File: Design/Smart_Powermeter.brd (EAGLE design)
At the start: 92 x 87 mm, 37 parts, among them J1 AUDIO_JACK_TRRSSMD_RA, J2 AUDIO_JACK_TRRSSMD_RA, J3 AUDIO_JACK_TRRSSMD_RA, J4 AUDIO_JACK_TRRSSMD_RA, J5 AUDIO_JACK_TRRSSMD_RA, J6 AUDIO_JACK_TRRSSMD_RA, J7 AUDIO_JACK_TRRSSMD_RA

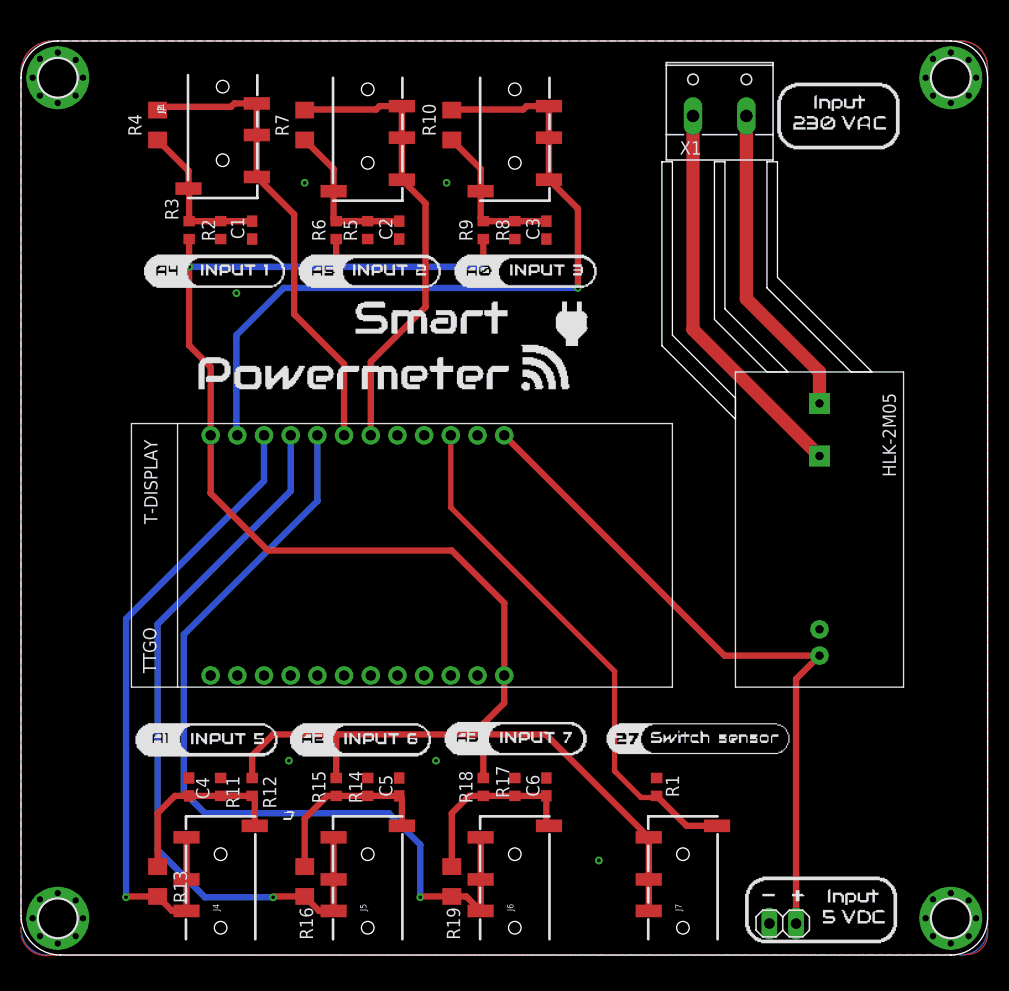
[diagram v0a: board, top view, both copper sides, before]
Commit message: Added design files of V2
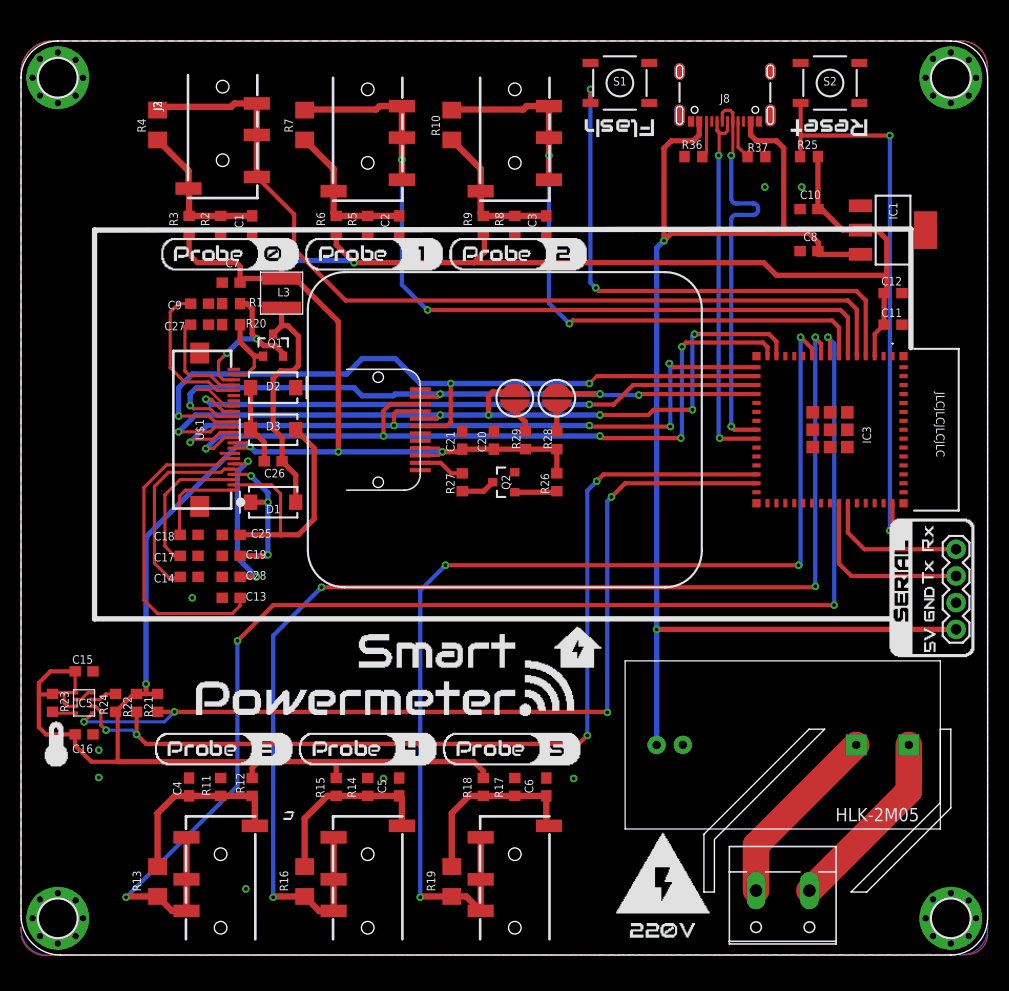
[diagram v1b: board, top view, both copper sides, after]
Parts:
- removed JP1: (no value), pinhead:1X02
- added C10, C12, C16, C20, C8: 10uF, rcl:C0603
- added C11, C15, C21: 0.1uF, rcl:C0603
- added C13, C14, C17, C18, C19, C25, C27, C28, C9: 1uF, rcl:C0603
- added C26, C7: 4.7uF, rcl:C0603
- added D1, D2, D3: SS14, SpaceDIY_semiconductors:SMA-DIODE
- added DISP1: DISP_LCD_GENERIC_SPI_1.69_WRAPUNDER, adafruit_display:TFT_1.69IN_240X280_12P
- added IC1: AMS1117-3.3, SparkFun-IC-Power:SOT223
- added IC3: ESP32-S2-MINI-1-N4R2, SpaceDIY_modules:ESP32S2MINI1N4R2
- added IC5: BMP280, SamacSys_Parts:8-PIN-METAL-LID-LGA
- added J8: USB-C, SparkFun-Connectors:USB-C-16P-4LAYER-ISOLATED
- added L3: 10uH, microbuilder:INDUCTOR_4X4MM_NR401
- added Q1: IRLML0100, Parts:SOT23-3
- added Q2: 2N7002, SparkFun-DiscreteSemi:SOT23-3
- added R20, R21, R22, R26, R28, R29: 10k, rcl:R0603
- added R23, R24: 4.7k, rcl:R0603
- added R25: 10K, rcl:R0603
- added R27: 10, rcl:R0603
- added R36, R37: 5.1k, rcl:R0603
- added S1: Flash, SpaceDIY_electromechanical:TACTILE_SWITCH_SMD_5.2MM
- added S2: Reset, SpaceDIY_electromechanical:TACTILE_SWITCH_SMD_5.2MM
- added SJ1, SJ2: SOLDERJUMPERROUND, SparkFun-Retired:SJ_ROUND
- H1: value (none) -> 92X84
- J7: value AUDIO_JACK_TRRSSMD_RA -> (none); device SparkFun-Connectors:AUDIO_JACK_3.5MM_TRRS_SMD_RA -> SparkFun-Connectors:1X04
- R1: value 10k -> 0.47
- U$1: value TTGO-T-DISPLAYFRAME -> E-PAPER-FPC_2; device TTGO-TDisplay:TTGO-T-DISPLAY-OL -> SpaceDIY_connectors:FPC-05FB-24PH20
- moved X1 75.2 mm to (72.5, 5.50), turned to 180 degrees
- moved R1 61.3 mm to (20.0, 62.0), turned to 180 degrees
- moved U$1 51.2 mm to (17.0, 50.0), turned to 270 degrees
- moved J7 39.7 mm to (89.0, 31.0)
- moved U$2 33.7 mm to (87.5, 28.0), turned to 180 degrees
- moved C1 0.50 mm to (22.0, 69.5)
- moved C2 0.50 mm to (36.0, 69.5)
- moved C3 0.50 mm to (50.0, 69.5)
- moved R2 0.50 mm to (19.0, 69.5)
- moved R3 0.50 mm to (16.0, 69.5)
- moved R5 0.50 mm to (33.0, 69.5)
- moved R6 0.50 mm to (30.0, 69.5)
- moved R8 0.50 mm to (47.0, 69.5)
- moved R9 0.50 mm to (44.0, 69.5)
- renumbered FRAME1 to H1
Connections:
- removed net M6: J6.RING1, J6.RING2, J6.TIP, R19.2, U$1.SVN-G39-A3
- removed net PB: J7.EARTH, R1.2, U$1.27-G27-A17
- removed net VG6: C6.1, J6.EARTH, R17.2, R18.1, R19.1
- new net BK_LIGHT: Q2.1, R26.1
- new net CC3: J8.B5, R36.2
- new net CC4: J8.A5, R37.2
- new net D+: IC3.24, J8.A6, J8.B6
- new net D-: IC3.23, J8.A7, J8.B7
- new net GDR: Q1.1, R20.1, U$1.23
- new net IO0: IC3.4, S1.3
- new net LEDK: DISP1.2, R27.2
- new net M0: IC3.5, J1.RING1, J1.RING2, J1.TIP, R4.2
- new net N$10: IC5.5, R23.2
- new net N$11: C9.2, U$1.20
- new net N$12: C13.2, U$1.7
- new net N$13: C14.2, U$1.5
- new net N$14: C17.2, U$1.3
- new net N$15: C18.2, U$1.1
- new net N$16: C26.2, D2.A, D3.C
- new net N$17: C26.1, D1.A, L3.P$1, Q1.3
- new net N$3: IC5.2, R24.2
- new net N$31: C27.2, U$1.21
- new net N$32: C28.2, U$1.6
- new net N$4: Q2.3, R27.1
- new net N$5: R28.1, SJ1.2
- new net N$6: R29.1, SJ2.2
- new net RESE: Q1.2, R1.1, U$1.22
- new net RST: IC3.45, R25.1, S2.3
- new net RX: IC3.40, J7.4
- new net SCL: IC3.29, IC5.4, R21.2
- new net SDA: IC3.28, IC5.3, R22.2
- new net SPI_BUSY: IC3.18, U$1.16
- new net SPI_CLK: DISP1.9, IC3.16, U$1.12
- new net SPI_CS: DISP1.8, IC3.14, SJ2.1, U$1.13
- new net SPI_MISO: DISP1.7, IC3.17, U$1.14
- new net SPI_MOSI: DISP1.10, IC3.15, U$1.11
- new net SPI_RST: DISP1.11, IC3.19, SJ1.1, U$1.15
- new net TX: IC3.39, J7.3
- new net VG0: C1.1, J1.EARTH, R2.2, R3.1, R4.1
- new net VGH: C19.1, D1.C, U$1.4
- new net VGL: C25.1, D3.A, U$1.2
- net 3.3V: now also C10.1, C11.1, C12.1, C15.1, C16.1, C20.1, C21.1, C7.1, DISP1.3, DISP1.4, IC1.2, IC3.3, IC5.6, IC5.8, L3.P$2, R21.1, R22.1, R23.1, R24.1, R25.2, R26.2, R28.2, R29.2, U$1.10, U$1.9; no longer J7.RING1, J7.RING2, J7.TIP, U$1.3V3_0, U$1.3V3_1
- net 5V: now also C8.1, IC1.3, J7.1, J8.VBUS1, J8.VBUS2; no longer JP1.2, U$1.5V
- net GND: now also C10.2, C11.2, C12.2, C13.1, C14.1, C15.2, C16.2, C17.1, C18.1, C19.2, C20.2, C21.2, C25.2, C27.1, C28.1, C7.2, C8.2, C9.1, D2.C, DISP1.1, DISP1.12, DISP1.5, DISP1.6, H1.B3,1, H1.B3,2, H1.B3,3, H1.B3,6, H1.P$1, H1.P$10, H1.P$11, H1.P$12, H1.P$13, H1.P$14, H1.P$15, H1.P$16, H1.P$17, H1.P$18, H1.P$19, H1.P$2, H1.P$20, H1.P$21, H1.P$22, H1.P$23, H1.P$24, H1.P$25, H1.P$26, H1.P$27, H1.P$28, H1.P$29, H1.P$3, H1.P$30, H1.P$31, H1.P$32, H1.P$4, H1.P$5, H1.P$6, H1.P$7, H1.P$8, H1.P$9, IC1.1, IC3.1, IC3.2, IC3.30, IC3.42, IC3.43, IC3.46, IC3.47, IC3.48, IC3.49, IC3.50, IC3.51, IC3.52, IC3.53, IC3.54, IC3.55, IC3.56, IC3.57, IC3.58, IC3.59, IC3.60, IC3.61, IC3.62, IC3.63, IC3.64, IC3.65, IC3.66, IC3.67, IC3.68, IC3.69, IC3.70, IC3.71, IC3.72, IC3.73, IC5.1, IC5.7, J7.2, J8.GND, J8.GND2, Q2.2, R1.2, R20.2, R36.1, R37.1, S1.1, S2.1, U$1.17, U$1.8; no longer JP1.1, R1.1, U$1.GND_0, U$1.GND_1, U$1.GND_2, U$1.GND_3, U$1.GND_4
- net M1: now also IC3.6, J2.RING1, J2.RING2, J2.TIP, R7.2; no longer J1.RING1, J1.RING2, J1.TIP, R4.2, U$1.32-G32-A4
- net M2: now also IC3.7, J3.RING1, J3.RING2, J3.TIP, R10.2; no longer J2.RING1, J2.RING2, J2.TIP, R7.2, U$1.33-G33-A5
- net M3: now also IC3.8, J4.RING1, J4.RING2, J4.TIP, R13.2; no longer J3.RING1, J3.RING2, J3.TIP, R10.2, U$1.SVP-G36-A0
- net M4: now also IC3.9, J5.RING1, J5.RING2, J5.TIP, R16.2; no longer J4.RING1, J4.RING2, J4.TIP, R13.2, U$1.37-G37
- net M5: now also IC3.10, J6.RING1, J6.RING2, J6.TIP, R19.2; no longer J5.RING1, J5.RING2, J5.TIP, R16.2, U$1.38-G38
- net N$1: now also U$2.AC2; no longer U$2.AC1
- net N$2: now also U$2.AC1; no longer U$2.AC2
- net VG1: now also C2.1, J2.EARTH, R5.2, R6.1, R7.1; no longer C1.1, J1.EARTH, R2.2, R3.1, R4.1
- net VG2: now also C3.1, J3.EARTH, R10.1, R8.2, R9.1; no longer C2.1, J2.EARTH, R5.2, R6.1, R7.1
- net VG3: now also C4.1, J4.EARTH, R11.2, R12.1, R13.1; no longer C3.1, J3.EARTH, R10.1, R8.2, R9.1
- net VG4: now also C5.1, J5.EARTH, R14.2, R15.1, R16.1; no longer C4.1, J4.EARTH, R11.2, R12.1, R13.1
- net VG5: now also C6.1, J6.EARTH, R17.2, R18.1, R19.1; no longer C5.1, J5.EARTH, R14.2, R15.1, R16.1
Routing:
- net 3.3V: track 164.0 -> 265.6 mm, vias 3 -> 6
- net SDA: track 0.00 -> 91.8 mm, vias 0 -> 4
- net SCL: track 0.00 -> 88.0 mm, vias 0 -> 4
- net M0: track 0.00 -> 85.4 mm
- net M6: track 82.2 -> 0.00 mm, vias 1 -> 0
- net SPI_CS: track 0.00 -> 78.7 mm, vias 0 -> 6
- net SPI_MOSI: track 0.00 -> 73.1 mm, vias 0 -> 5
- net SPI_MISO: track 0.00 -> 72.3 mm, vias 0 -> 3
- net SPI_CLK: track 0.00 -> 69.1 mm, vias 0 -> 5
- net SPI_RST: track 0.00 -> 66.5 mm, vias 0 -> 4
- net 5V: track 65.1 -> 124.5 mm, vias 0 -> 2
- net SPI_BUSY: track 0.00 -> 56.5 mm, vias 0 -> 2
- net M3: track 71.8 -> 128.0 mm, vias 1 -> 4
- net M4: track 62.8 -> 117.5 mm, vias 1 -> 4
- net RST: track 0.00 -> 53.9 mm, vias 0 -> 2
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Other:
- board text added: "JLCJLCJLCJLC"

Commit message: Updated design files
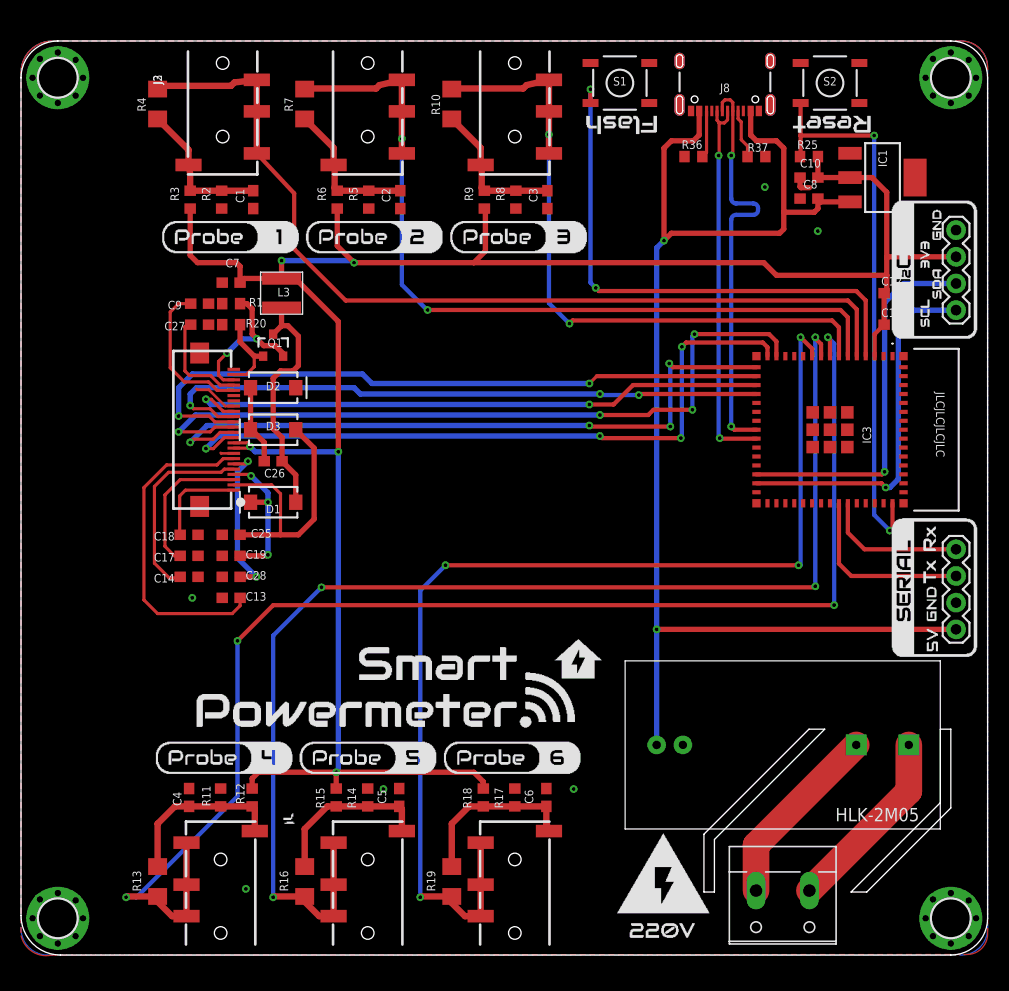
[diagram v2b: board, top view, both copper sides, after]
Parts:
- removed C15, C21: 0.1uF, rcl:C0603
- removed C16, C20: 10uF, rcl:C0603
- removed DISP1: DISP_LCD_GENERIC_SPI_1.69_WRAPUNDER, adafruit_display:TFT_1.69IN_240X280_12P
- removed IC5: BMP280, SamacSys_Parts:8-PIN-METAL-LID-LGA
- removed Q2: 2N7002, SparkFun-DiscreteSemi:SOT23-3
- removed R21, R22, R26, R28, R29: 10k, rcl:R0603
- removed R23, R24: 4.7k, rcl:R0603
- removed R27: 10, rcl:R0603
- removed SJ1, SJ2: SOLDERJUMPERROUND, SparkFun-Retired:SJ_ROUND
- added J9: (no value), SparkFun-Connectors:1X04
- moved IC1 5.10 mm to (82.0, 74.0)
- moved C8 5.00 mm to (75.0, 72.0)
- moved C10 3.00 mm to (75.0, 74.0)
- moved J2 2.50 mm to (33.0, 86.5)
- moved J3 2.50 mm to (47.0, 86.5)
- moved C1 2.40 mm to (22.1, 71.9)
- moved C2 2.40 mm to (36.1, 71.9)
- moved C3 2.40 mm to (50.1, 71.9)
- moved R2 2.40 mm to (19.1, 71.9)
- moved R3 2.40 mm to (16.1, 71.9)
- moved R5 2.40 mm to (33.1, 71.9)
- moved R6 2.40 mm to (30.1, 71.9)
- moved R8 2.40 mm to (47.1, 71.9)
- moved R9 2.40 mm to (44.1, 71.9)
- moved J1 2.25 mm to (19.2, 86.5)
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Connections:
- removed net BK_LIGHT: Q2.1, R26.1
- removed net LEDK: DISP1.2, R27.2
- removed net M0: IC3.5, J1.RING1, J1.RING2, J1.TIP, R4.2
- removed net N$10: IC5.5, R23.2
- removed net N$3: IC5.2, R24.2
- removed net N$4: Q2.3, R27.1
- removed net N$5: R28.1, SJ1.2
- removed net N$6: R29.1, SJ2.2
- new net M6: IC3.10, J6.RING1, J6.RING2, J6.TIP, R19.2
- net 3.3V: now also J9.2; no longer C15.1, C16.1, C20.1, C21.1, DISP1.3, DISP1.4, IC5.6, IC5.8, R21.1, R22.1, R23.1, R24.1, R26.2, R28.2, R29.2
- net GND: now also J9.1; no longer C15.2, C16.2, C20.2, C21.2, DISP1.1, DISP1.12, DISP1.5, DISP1.6, IC5.1, IC5.7, Q2.2
- net M1: now also IC3.5, J1.RING1, J1.RING2, J1.TIP, R4.2; no longer IC3.6, J2.RING1, J2.RING2, J2.TIP, R7.2
- net M2: now also IC3.6, J2.RING1, J2.RING2, J2.TIP, R7.2; no longer IC3.7, J3.RING1, J3.RING2, J3.TIP, R10.2
- net M3: now also IC3.7, J3.RING1, J3.RING2, J3.TIP, R10.2; no longer IC3.8, J4.RING1, J4.RING2, J4.TIP, R13.2
- net M4: now also IC3.8, J4.RING1, J4.RING2, J4.TIP, R13.2; no longer IC3.9, J5.RING1, J5.RING2, J5.TIP, R16.2
- net M5: now also IC3.9, J5.RING1, J5.RING2, J5.TIP, R16.2; no longer IC3.10, J6.RING1, J6.RING2, J6.TIP, R19.2
- net SCL: now also J9.4; no longer IC5.4, R21.2
- net SDA: now also J9.3; no longer IC5.3, R22.2
- net SPI_CLK: no longer DISP1.9
- net SPI_CS: no longer DISP1.8, SJ2.1
- net SPI_MISO: no longer DISP1.7
- net SPI_MOSI: no longer DISP1.10
- net SPI_RST: no longer DISP1.11, SJ1.1
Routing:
- net M6: track 0.00 -> 104.3 mm, vias 0 -> 4
- net M0: track 85.4 -> 0.00 mm
- net M3: track 128.0 -> 64.1 mm, vias 4 -> 2
- net 3.3V: track 265.6 -> 206.4 mm, vias 6 -> 5
- net SDA: track 91.8 -> 36.0 mm, vias 4 -> 1
- net SCL: track 88.0 -> 34.7 mm, vias 4 -> 1
- net M2: track 62.0 -> 77.8 mm
- net M5: track 103.7 -> 118.0 mm
- net M1: track 75.7 -> 87.6 mm, vias 2 -> 0
- net M4: track 117.5 -> 129.1 mm
- net SPI_MISO: track 72.3 -> 64.4 mm, vias 3 -> 2
- net SPI_CS: track 78.7 -> 72.0 mm, vias 6 -> 4
- net SPI_RST: track 66.5 -> 60.2 mm, vias 4 -> 3
- net SPI_MOSI: track 73.1 -> 67.0 mm, vias 5 -> 4
- net LEDK: track 4.41 -> 0.00 mm
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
